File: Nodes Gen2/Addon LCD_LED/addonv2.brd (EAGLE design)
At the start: 55.5 x 48 mm, 59 parts, among them J3 22-05-7038-03, J4 22-05-7048-04, J5 22-05-7048-04

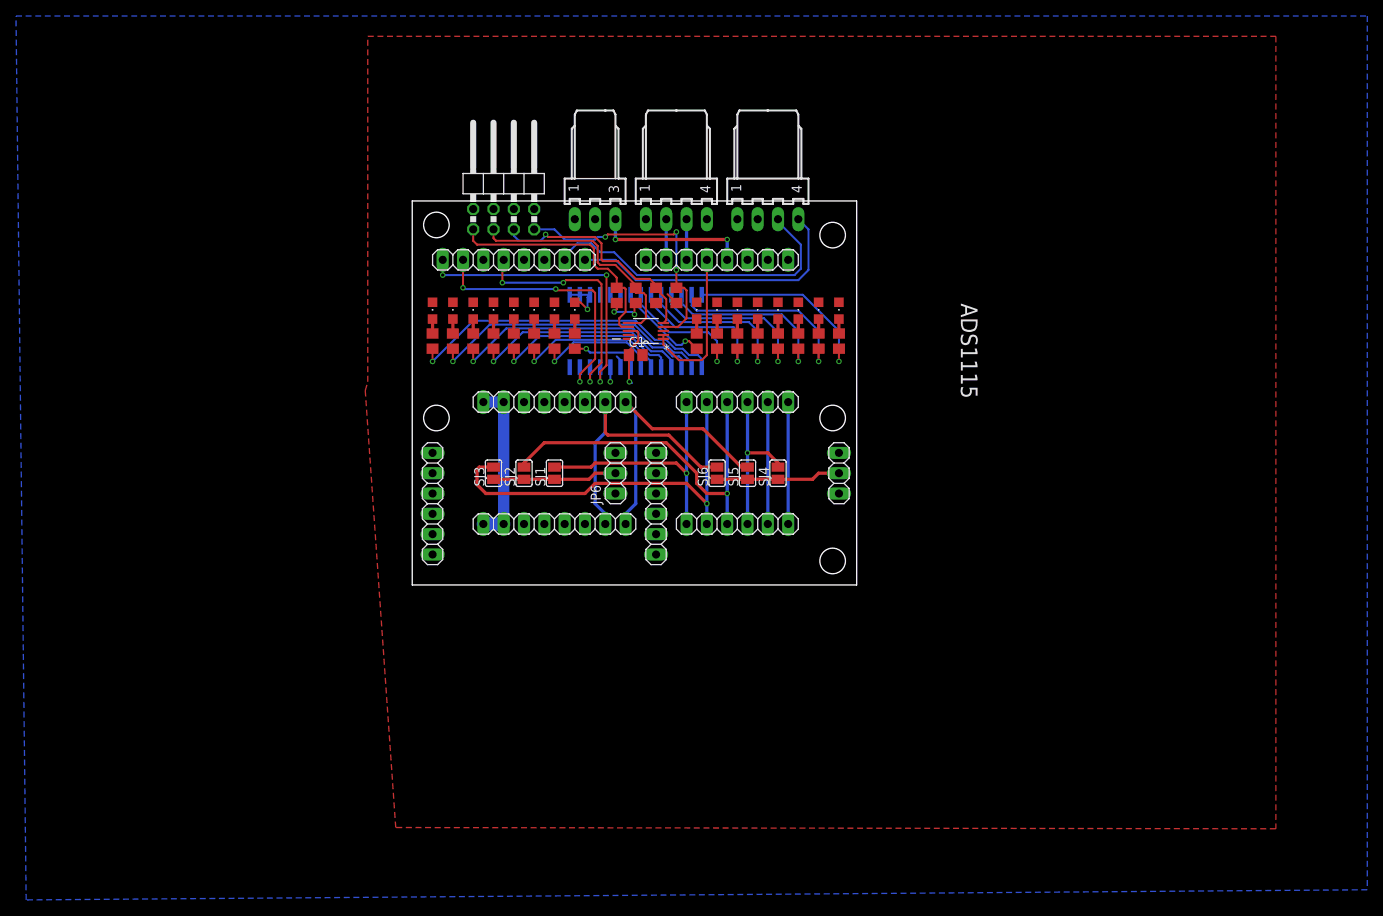
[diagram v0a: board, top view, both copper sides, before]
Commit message: gen 2 dev + bom
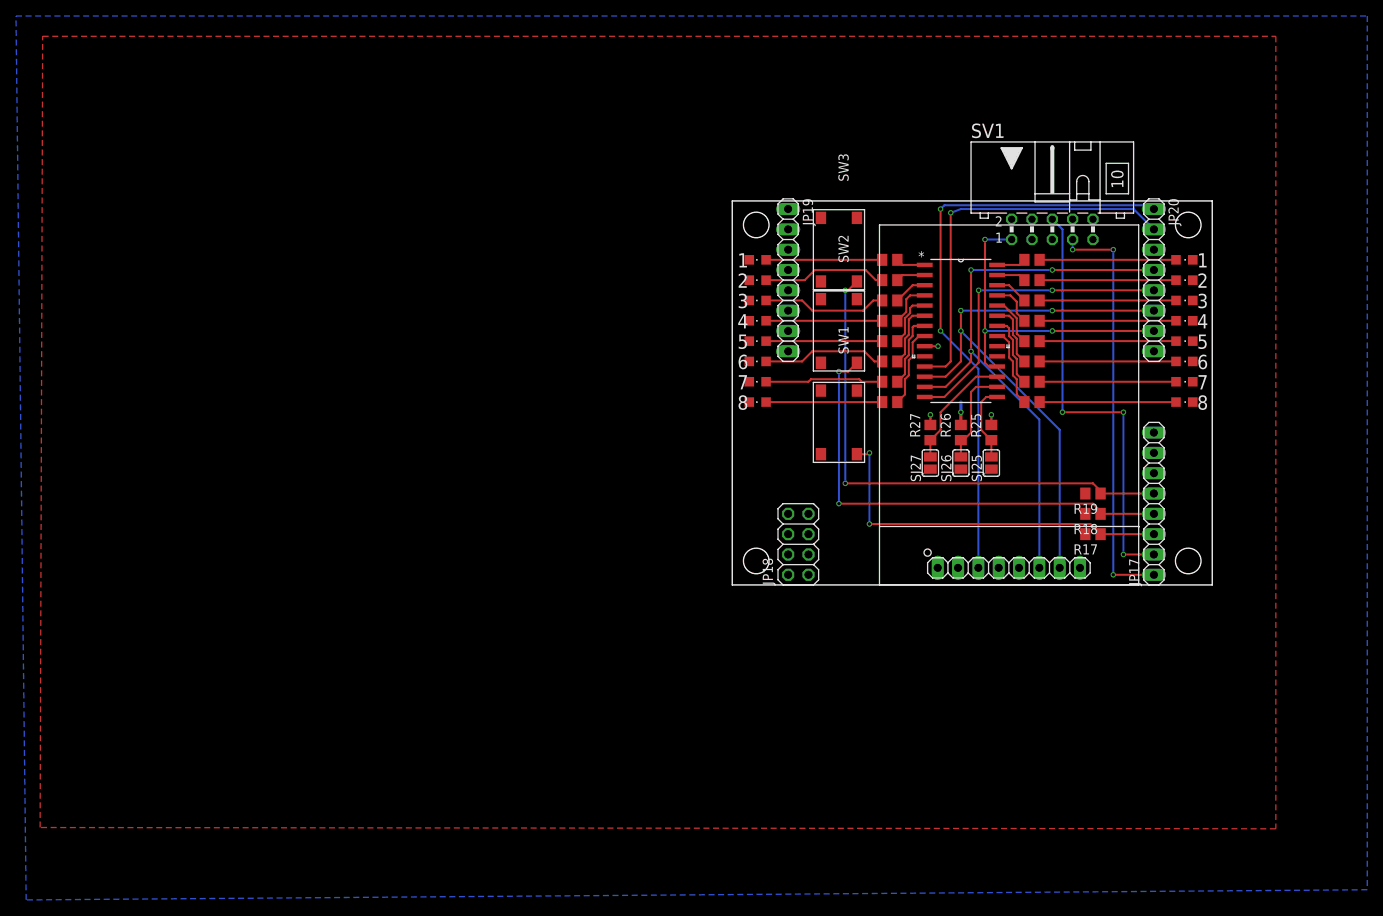
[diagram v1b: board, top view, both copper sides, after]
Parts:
- removed ADS1115: ADS1115IDGST, schlager_ics:SOP50P490X110-10N
- removed C1: 100n, schlager_passiv:C0805
- removed J3: 22-05-7038-03, con-molex:7395-03
- removed J4, J5: 22-05-7048-04, con-molex:7395-04
- removed JP1, JP11, JP3, JP5: (no value), pinhead:1X08
- removed JP12, JP6: (no value), pinhead:1X03
- removed JP2, JP4, JP7, JP8: (no value), pinhead:1X06
- removed JP9: (no value), pinhead:2X04/90
- removed R20, R21, R22: 10k, rcl:R0805
- removed SJ1, SJ2, SJ3, SJ4, SJ5, SJ6: (no value), jumper:SJ
- added JP17, JP19, JP20: (no value), pinhead:1X08
- added JP18: (no value), pinhead:2X04
- added R17, R18, R25, R26, R27: 10k, rcl:R0805
- added SJ25, SJ26, SJ27: (no value), jumper:SJ
- added SV1: (no value), X_Pfostenstecker:ML10L
- added SW1, SW2, SW3: 430152043826, Wuerth_Elektronik_Switch:430152043826
- added U$3: 1.44-128X128, schlager_modules:1.44-128X128
- moved R19 64.5 mm to (85.1, 11.4), turned to 180 degrees
- moved LED16 62.0 mm to (96.5, 22.9), turned to 270 degrees
- moved LED14 59.1 mm to (96.5, 25.4), turned to 270 degrees
- moved R9 58.0 mm to (59.7, 40.6), turned to 180 degrees
- moved LED12 56.2 mm to (96.5, 27.9), turned to 270 degrees
- moved R10 55.1 mm to (59.7, 38.1), turned to 180 degrees
- moved LED10 53.5 mm to (96.5, 30.5), turned to 270 degrees
- moved R11 52.3 mm to (59.7, 35.6), turned to 180 degrees
- moved LED8 50.8 mm to (96.5, 33.0), turned to 270 degrees
- moved R12 49.6 mm to (59.7, 33.0), turned to 180 degrees
- moved LED6 48.3 mm to (96.5, 35.6), turned to 270 degrees
- moved R13 47.0 mm to (59.7, 30.5), turned to 180 degrees
- moved LED4 45.9 mm to (96.5, 38.1), turned to 270 degrees
- moved R14 44.5 mm to (59.7, 27.9), turned to 180 degrees
- moved LED2 43.6 mm to (96.5, 40.6), turned to 270 degrees
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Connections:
- removed net A4_SDA2: JP4.5, JP7.5
- removed net A5_SCL2: JP4.6, JP7.6
- removed net AREF: JP11.6
- removed net DR1: JP4.1, JP7.1, SJ1.2
- removed net DR2: JP4.2, JP7.2, SJ3.2
- removed net DR3: JP4.3, JP7.3, SJ2.2
- removed net DR4: JP4.4, JP7.4, SJ4.2
- removed net DR5: JP3.8, JP5.8, SJ5.2
- removed net DR6: JP3.7, JP5.7, SJ6.2
- removed net N$33: JP6.2, SJ1.1, SJ2.1, SJ3.1
- removed net N$34: JP12.2, SJ4.1, SJ5.1, SJ6.1
- removed net SCL: ADS1115.10
- removed net SDA: ADS1115.9
- new net A6: JP19.7
- new net A7: JP19.8
- new net D8_SS: JP20.1, U$3.3
- new net D9_SS: JP20.2, U$1.11
- new net N$38: R25.1, SJ25.2, U$1.15
- new net N$39: R26.1, SJ26.2, U$1.16
- new net N$40: R27.1, SJ27.2, U$1.17
- new net PE2: SV1.2
- new net RESERVE2: JP20.8
- new net RESET_LCD: U$3.4
- new net TCK: SV1.4
- new net TDI: SV1.8
- new net TDO: SV1.5
- new net TMS: SV1.3
- net A0: now also JP19.1; no longer ADS1115.4, JP9.7, R22.2
- net A1: now also JP19.2; no longer ADS1115.5, JP9.5, R21.2
- net A2: now also JP19.3; no longer ADS1115.6, JP9.3, R20.2
- net A3: now also JP19.4; no longer ADS1115.7, JP9.1, R19.2
- net A4_SDA: now also JP19.5; no longer J4.3, JP11.7
- net A5_SCL: now also JP19.6; no longer J4.4, JP11.8
- net D10_SS: now also JP20.3; no longer JP11.1, U$1.11
- net D11_MOSI: now also JP20.4, U$3.6; no longer JP11.2
- net D12_MISO: now also JP20.5, U$1.14; no longer JP11.3
- net D13_SCK: now also JP20.6, U$3.7; no longer JP11.4
- net D2: now also JP17.3, R17.1, SW1.3; no longer JP1.3
- net D3: now also JP17.4, R18.1, SW2.3; no longer J3.3, JP1.4
- net D4: now also JP17.5, R19.1, SW3.3; no longer ADS1115.2, JP1.5
- net D5: now also JP17.6; no longer J5.3, JP1.6
- net D6: now also JP17.7; no longer J5.2, JP1.7
- net D7: now also JP17.8; no longer JP1.8
- net GND: now also JP18.3, JP18.4, SJ25.1, SJ26.1, SJ27.1, SV1.10, SW1.4, SW2.4, SW3.4, U$3.2; no longer ADS1115.1, ADS1115.3, C1.2, J3.1, J4.2, J5.1, JP11.5, JP12.1, JP3.3, JP3.4, JP5.3, JP5.4, JP6.1, R19.1, R20.1, R21.1, R22.1, U$1.15, U$1.16, U$1.17
- net P24P: now also JP18.7, JP18.8; no longer JP3.1, JP3.2, JP5.1, JP5.2
- net P5V: now also JP18.1, JP18.2, R17.2, R18.2, R19.2, R25.2, R26.2, R27.2, SV1.9, U$3.1, U$3.8; no longer ADS1115.8, C1.1, J3.2, J4.1, J5.4, JP12.3, JP3.5, JP3.6, JP5.5, JP5.6, JP6.3, JP9.2, JP9.4, JP9.6, JP9.8
- net RESET: now also JP20.7, SV1.1
- net RX: now also JP17.1, SV1.7; no longer JP1.1
- net TX: now also JP17.2, SV1.6; no longer JP1.2
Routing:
- net D8_SS: track 0.00 -> 73.9 mm, vias 0 -> 2
- net TX: track 0.00 -> 53.9 mm, vias 0 -> 3
- net RX: track 0.00 -> 52.1 mm, vias 0 -> 3
- net DR2: track 50.1 -> 0.00 mm, vias 1 -> 0
- net D9_SS: track 0.00 -> 48.6 mm, vias 0 -> 1
- net D2: track 0.00 -> 46.6 mm, vias 0 -> 2
- net D4: track 19.6 -> 65.3 mm, vias 0 -> 2
- net DR3: track 45.6 -> 0.00 mm, vias 1 -> 0
- net RESET: track 0.00 -> 41.5 mm, vias 0 -> 3
- net D3: track 19.0 -> 59.3 mm
- net D13_SCK: track 30.3 -> 70.5 mm
- net A4_SDA: track 40.0 -> 0.00 mm
- net D12_MISO: track 0.00 -> 39.5 mm, vias 0 -> 2
- net D11_MOSI: track 34.0 -> 72.0 mm
- net D10_SS: track 37.9 -> 0.00 mm, vias 3 -> 0
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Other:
- board size 55.5 x 48 mm -> 60 x 48 mm
- board text added: "1"
- board text added: "2"
- board text added: "3"
- board text added: "4"
- board text added: "5"
- board text added: "6"
- board text added: "7"
- board text added: "8"
